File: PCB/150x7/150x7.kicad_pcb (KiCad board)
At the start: 2 copper layers, 14.5 x 14.5 mm, 51 parts, among them J1 Conn_01x03, J2 Conn_01x03

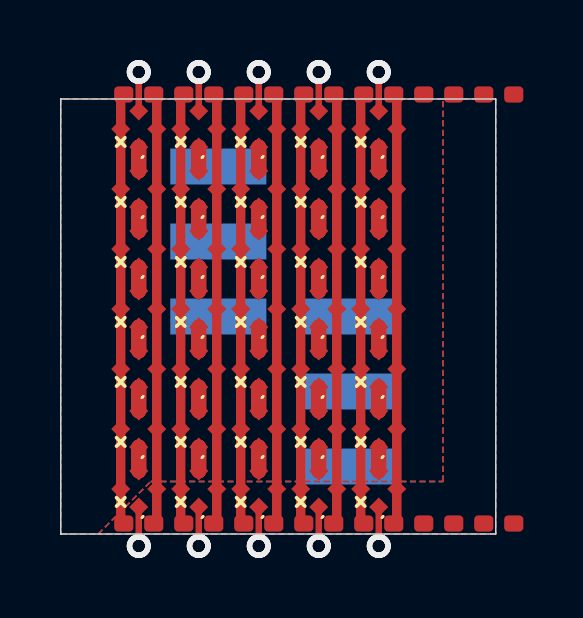
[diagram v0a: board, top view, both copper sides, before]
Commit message: New layout
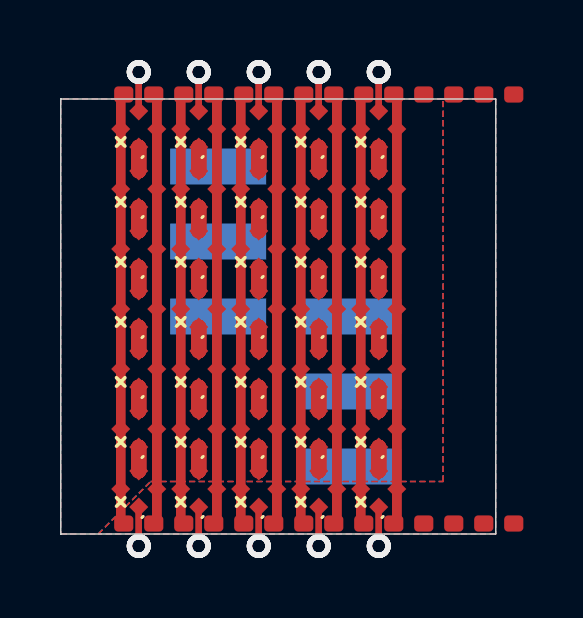
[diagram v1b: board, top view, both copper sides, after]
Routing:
- net (no net): track 359.9 -> 539.8 mm, vias 20 -> 30
